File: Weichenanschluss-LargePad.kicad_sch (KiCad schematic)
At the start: 36 parts, among them J1 A1.1, J1001 Conn_01x01, J11 +V, J12 fb1, J13 fb2, J2 A1.2, J22 Za, J23 H, J25 g, J26 a, J27 Tg, J28 Ta, J29 GND, J3 Aux1, J30 GND, J31 +12, J32 Rü1, J33 Rü2, J4 Aux2, J41 g, J42 a, J43 +12V, J44 GND, J5 A2.1, J51 g, J52 a, J53 +12V, J54 GND, J6 A2.2, J7 Prz1, J8 Prz2, J9 -V, U1001 ULN2803A

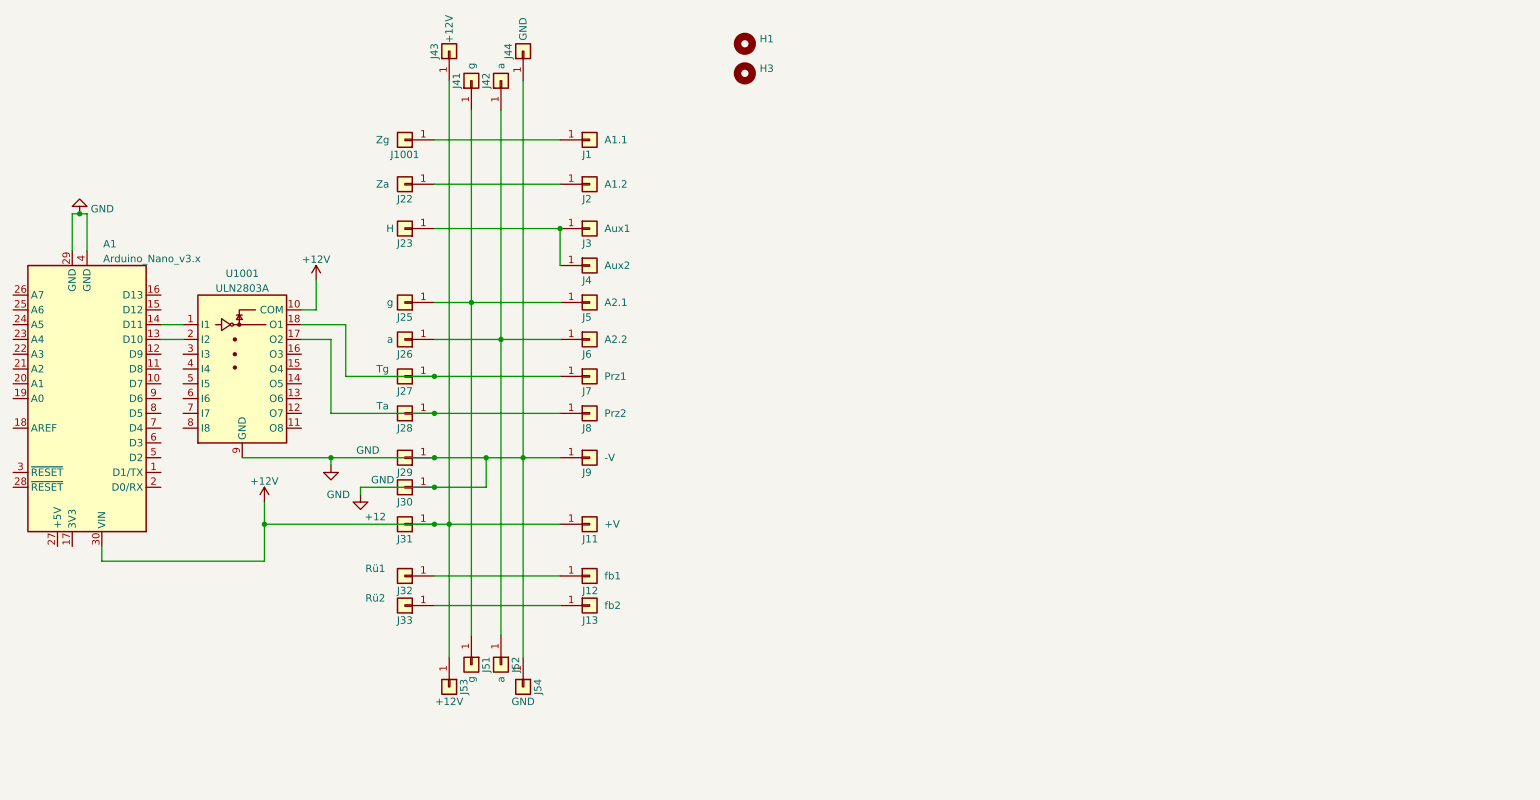
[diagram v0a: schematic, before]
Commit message: Kicad 10
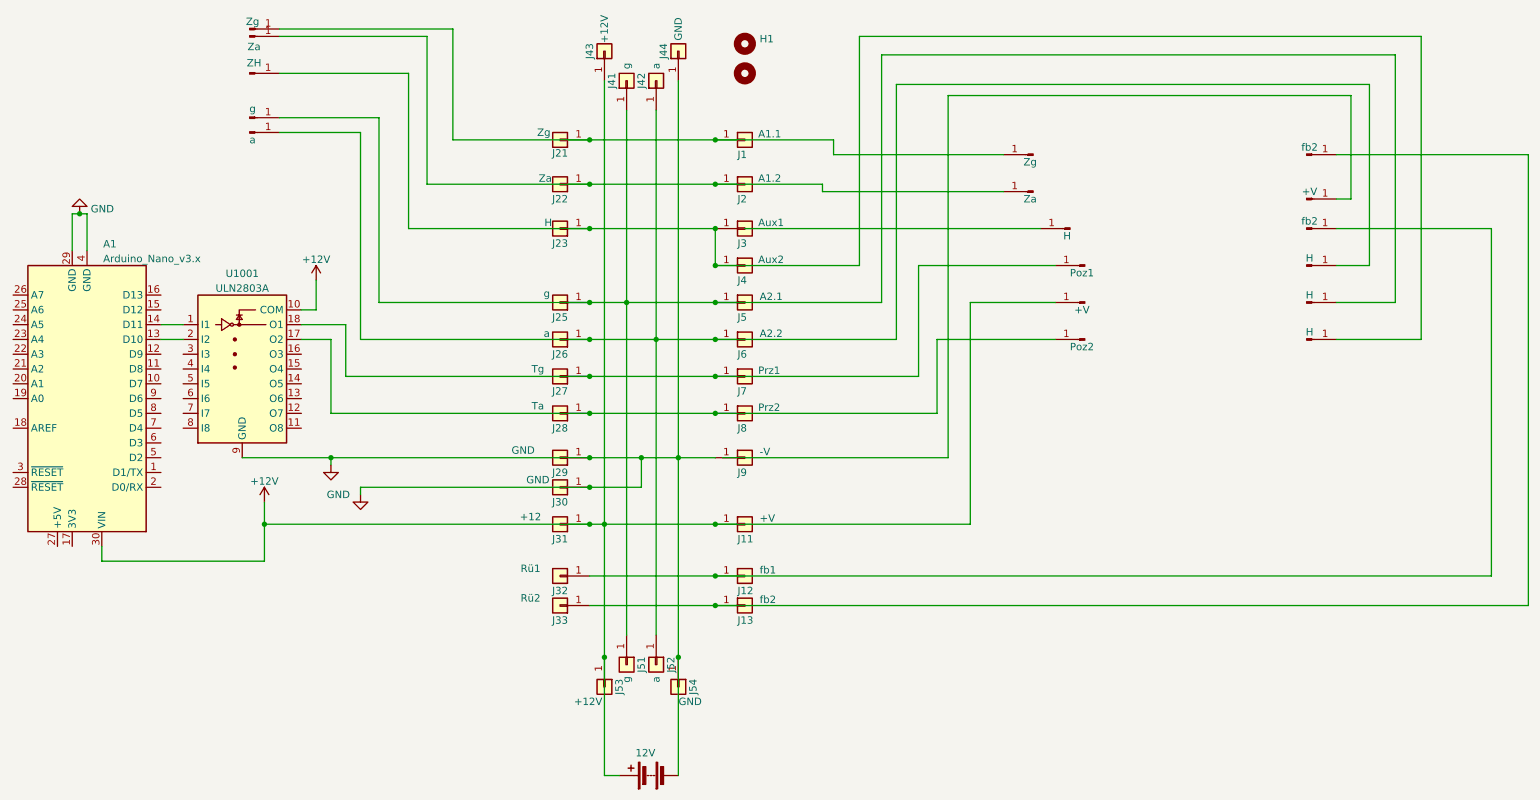
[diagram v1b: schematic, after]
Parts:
- added BT1001: 12V, symbol Device:Battery
- added J1001, J1006: Zg, symbol Connector:Conn_01x01_Pin
- added J1002, J1007: Za, symbol Connector:Conn_01x01_Pin
- added J1003: ZH, symbol Connector:Conn_01x01_Pin
- added J1004: g, symbol Connector:Conn_01x01_Pin
- added J1005: a, symbol Connector:Conn_01x01_Pin
- added J1008, J1012, J1013, J1014: H, symbol Connector:Conn_01x01_Pin
- added J1009: Poz1, symbol Connector:Conn_01x01_Pin
- added J1010, J1015: +V, symbol Connector:Conn_01x01_Pin
- added J1011: Poz2, symbol Connector:Conn_01x01_Pin
- added J1016, J1017: fb2, symbol Connector:Conn_01x01_Pin
- J21: renamed from J1001; value Conn_01x01 -> Zg
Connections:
- net +12V: now also BT1001.1 (+), J1010.1 (Pin_1)
- net GND: now also BT1001.2 (-)
- net at J13.1 (Pin_1), J33.1 (Pin_1): now also J1017.1 (Pin_1)
- net at J26.1 (Pin_1), J42.1 (Pin_1), J52.1 (Pin_1)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: now also J1005.1 (Pin_1), J1014.1 (Pin_1)
- net at J12.1 (Pin_1), J32.1 (Pin_1): now also J1016.1 (Pin_1)
- net at J27.1 (Pin_1), J7.1 (Pin_1), U1001.18 (O1): now also J1009.1 (Pin_1)
- net at J1.1 (Pin_1), J21.1 (Pin_1): now also J1001.1 (Pin_1), J1006.1 (Pin_1)
- net at J23.1 (Pin_1), J3.1 (Pin_1), J4.1 (Pin_1): now also J1003.1 (Pin_1), J1012.1 (Pin_1)
- net at J25.1 (Pin_1), J41.1 (Pin_1), J5.1 (Pin_1)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: now also J1004.1 (Pin_1), J1013.1 (Pin_1)
- net at J28.1 (Pin_1), J8.1 (Pin_1), U1001.17 (O2): now also J1011.1 (Pin_1)
- net at J2.1 (Pin_1), J22.1 (Pin_1): now also J1002.1 (Pin_1), J1007.1 (Pin_1)
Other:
- moved on the sheet: J1, J11, J12, J13, J2, J21, J22, J23, J25, J26, J27, J28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
